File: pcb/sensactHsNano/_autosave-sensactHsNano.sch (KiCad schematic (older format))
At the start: 29 parts, among them J1 PROG, J2 SensactBus, J3 CAN+24V, J6 1wire, SW1 TERM, SW2 Prog, SW3 Reset, U3 ESP32, U4 DS2482, U5 SN65HVD230

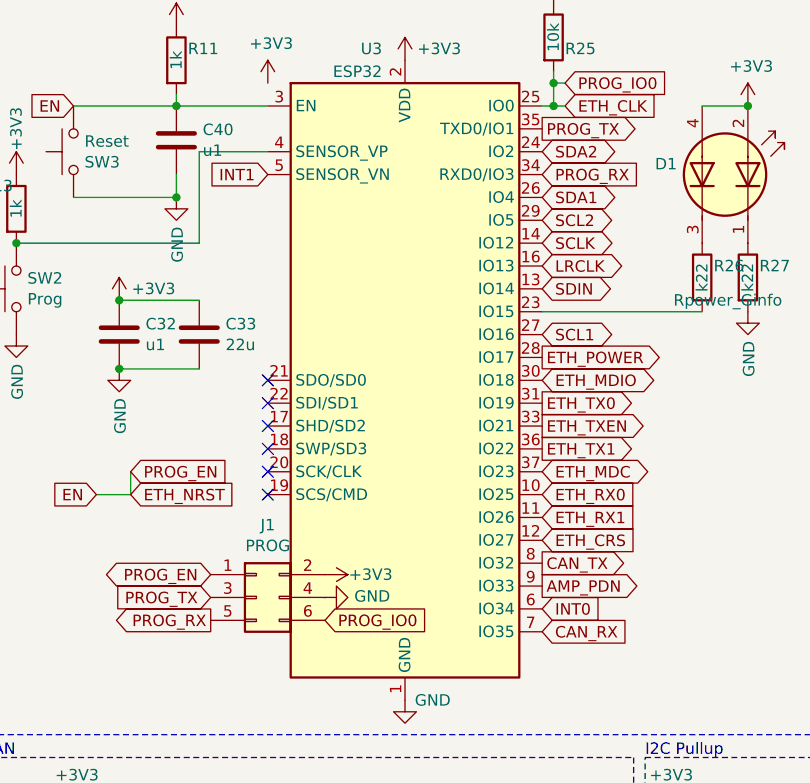
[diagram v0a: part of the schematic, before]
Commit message: Updated sensactHsNano
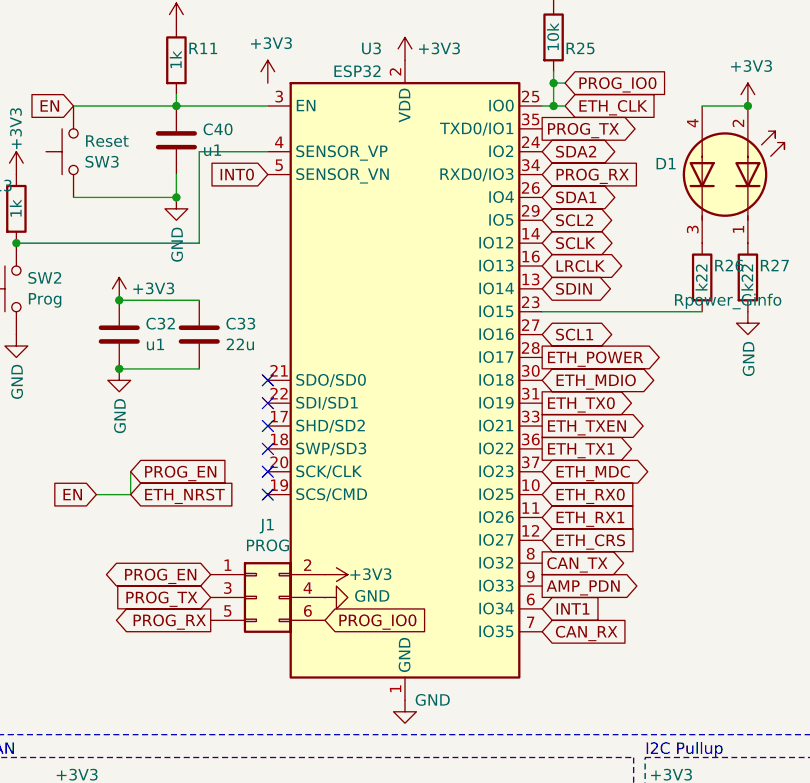
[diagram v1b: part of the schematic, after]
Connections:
- net INT0: now also U3.5 (SENSOR_VN); no longer U3.6 (IO34)
- net INT1: now also U3.6 (IO34); no longer U3.5 (SENSOR_VN)
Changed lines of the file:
@@
 Text GLabel 5050 5800 2    50   Output ~ 0
 INT1
+Text GLabel 1750 1500 0    50   Input ~ 0
+INT0
 Text GLabel 2950 3400 2    50   Input ~ 0
-INT0
-Text GLabel 1750 1500 0    50   Input ~ 0
 INT1
 Wire Wire Line
